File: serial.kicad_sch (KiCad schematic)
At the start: 9 parts

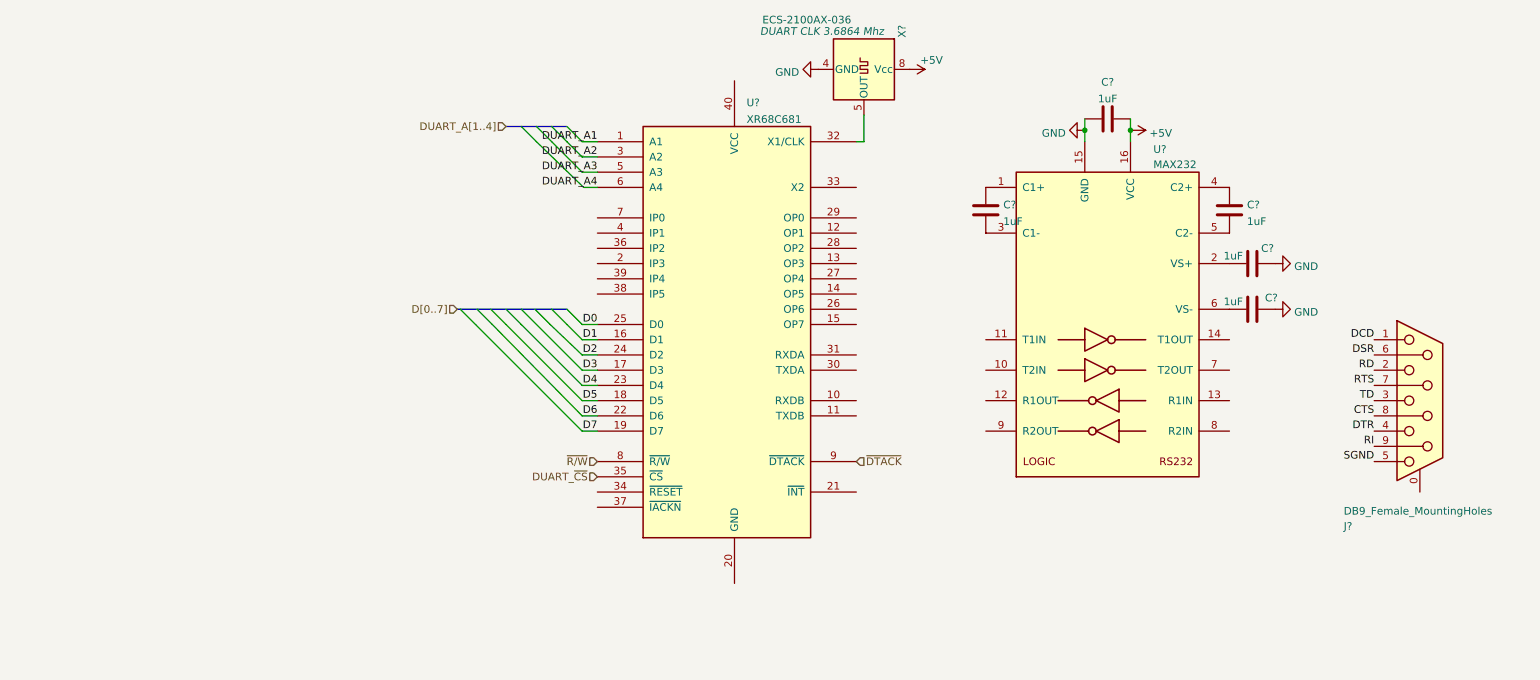
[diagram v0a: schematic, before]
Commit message: Final PCB Layout
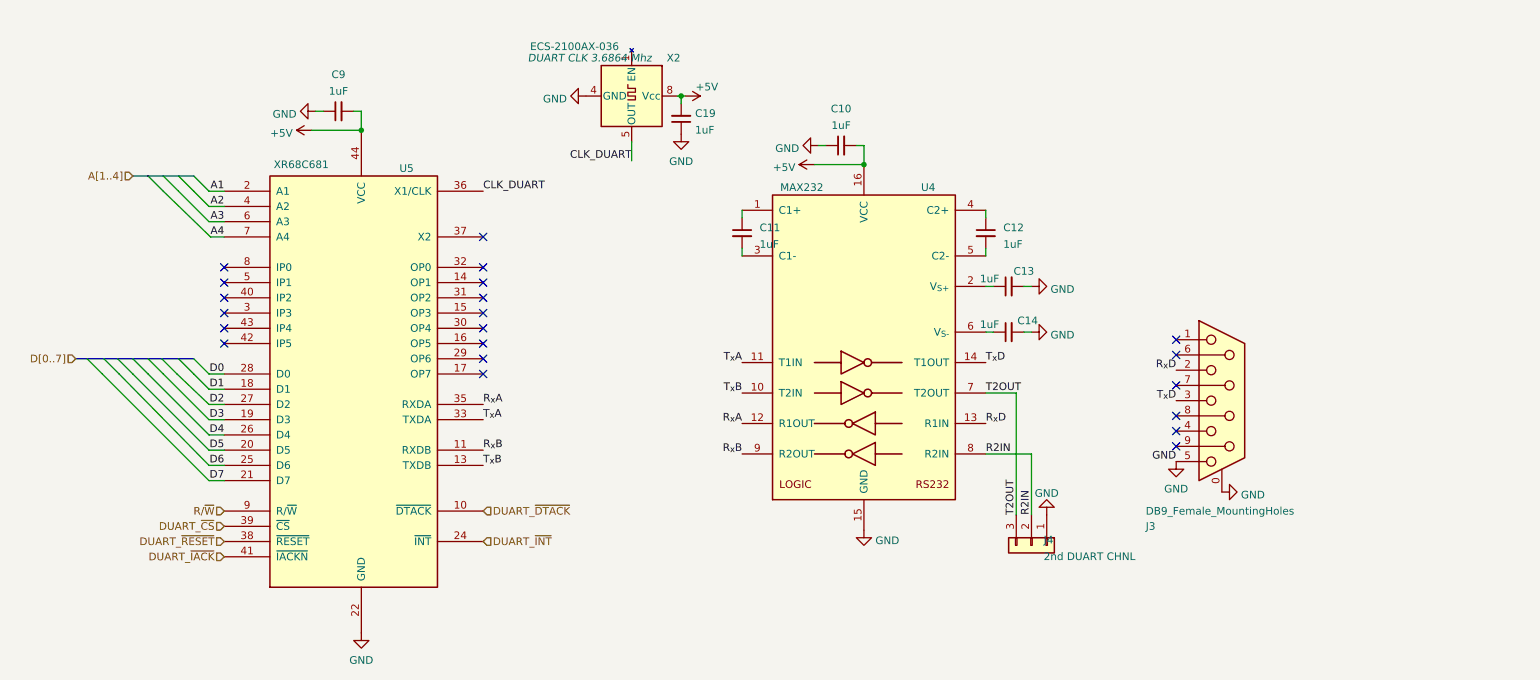
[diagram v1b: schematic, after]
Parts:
- removed C?: 1uF, Capacitor_SMD:C_0805_2012Metric_Pad1.18x1.45mm_HandSolder, symbol Device:C
- added C10, C19, C9: 1uF, Capacitor_SMD:C_0805_2012Metric_Pad1.18x1.45mm_HandSolder, symbol Device:C_Small
- added J4: 2nd DUART CHNL, Connector_PinHeader_2.54mm:PinHeader_1x03_P2.54mm_Vertical, symbol Connector_Generic:Conn_01x03
- C11, C12, C13, C14: renamed from C?; symbol Device:C -> Device:C_Small
- U5: renamed from U?; footprint Package_LCC:PLCC-44_SMD-Socket -> Package_LCC:PLCC-44_THT-Socket; symbol Interface_UART:68C681 -> MCD_Symbols:XR68C681
- X2: renamed from X?; symbol Oscillator:CXO_DIP8 -> MCD_Symbols:ECS_CLK_DIP8
- gave numbers to parts that had none: 2
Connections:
- net RD is gone; now on net R_{x}D: J3.2
- net SGND is gone; now on net GND: J3.5
- net TD is gone; now on net T_{x}D: J3.3
- net +5V: now also U5.44 (VCC), C10.2, C19.2, C9.2
- net D0: now also U5.28 (D0); no longer U5.25 (D0)
- net D1: now also U5.18 (D1); no longer U5.16 (D1)
- net D2: now also U5.27 (D2); no longer U5.24 (D2)
- net D3: now also U5.19 (D3); no longer U5.17 (D3)
- net D4: now also U5.26 (D4); no longer U5.23 (D4)
- net D5: now also U5.20 (D5); no longer U5.18 (D5)
- net D6: now also U5.25 (D6); no longer U5.22 (D6)
- net D7: now also U5.21 (D7); no longer U5.19 (D7)
- net DUART_~{CS}: now also U5.39 (~{CS}); no longer U5.35 (~{CS})
- net GND: now also J3.0 (PAD), U5.22 (GND), C10.1, C19.1, C9.1, J4.1 (Pin_1)
- net T_{x}B: now reaches U4.10 (T2IN)
- net T_{x}B: now also U5.13 (TXDB)
- net T_{x}A: now reaches U4.11 (T1IN)
- net T_{x}A: now also U5.33 (TXDA)
- net R_{x}A: now reaches U4.12 (R1OUT)
- net R_{x}A: now also U5.35 (RXDA)
- net R_{x}D: now reaches U4.13 (R1IN)
- net T_{x}D: now reaches U4.14 (T1OUT)
- net T2OUT: now reaches U4.7 (T2OUT)
- net T2OUT: now also J4.3 (Pin_3)
- net R2IN: now reaches U4.8 (R2IN)
- net R2IN: now also J4.2 (Pin_2)
- net R_{x}B: now reaches U4.9 (R2OUT)
- net R_{x}B: now also U5.11 (RXDB)
- net DUART_~{DTACK}: now reaches U5.10 (~{DTACK})
- net A1: now reaches U5.2 (A1)
- net at U5.32 (OP0): no longer X2.5 (OUT)
- net CLK_DUART: now reaches U5.36 (X1/CLK)
- net CLK_DUART: now also X2.5 (OUT)
- net DUART_~{RESET}: now reaches U5.38 (~{RESET})
- net A2: now reaches U5.4 (A2)
- net A4: now reaches U5.7 (A4)
- net CTS: no longer names the net of J3.8
- net DCD: no longer names the net of J3.1
- net DSR: no longer names the net of J3.6
- net DTR: no longer names the net of J3.4
- net DUART_A1: no longer names the net of U5.1 (NC)
- net DUART_A2: no longer names the net of U5.3 (IP3)
- net DUART_A3: no longer names the net of U5.5 (IP1)
- net DUART_A4 renamed A3
- net RI: no longer names the net of J3.9
- net RTS: no longer names the net of J3.7
- net ~{DTACK} renamed R/~{W}
- net ~{R/W}: no longer names the net of U5.8 (IP0)
- new net DUART_~{IACK}: U5.41 (~{IACKN})
- new net DUART_~{INT}: U5.24 (~{INT})
- no-connect marks 0 -> 21
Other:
- moved on the sheet: C11, C12, C13, C14, J3, U4, U5
